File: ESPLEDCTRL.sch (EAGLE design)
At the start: 6 parts, among them J1 22-27-2031-03, X3 ZX62D-B-5PA8

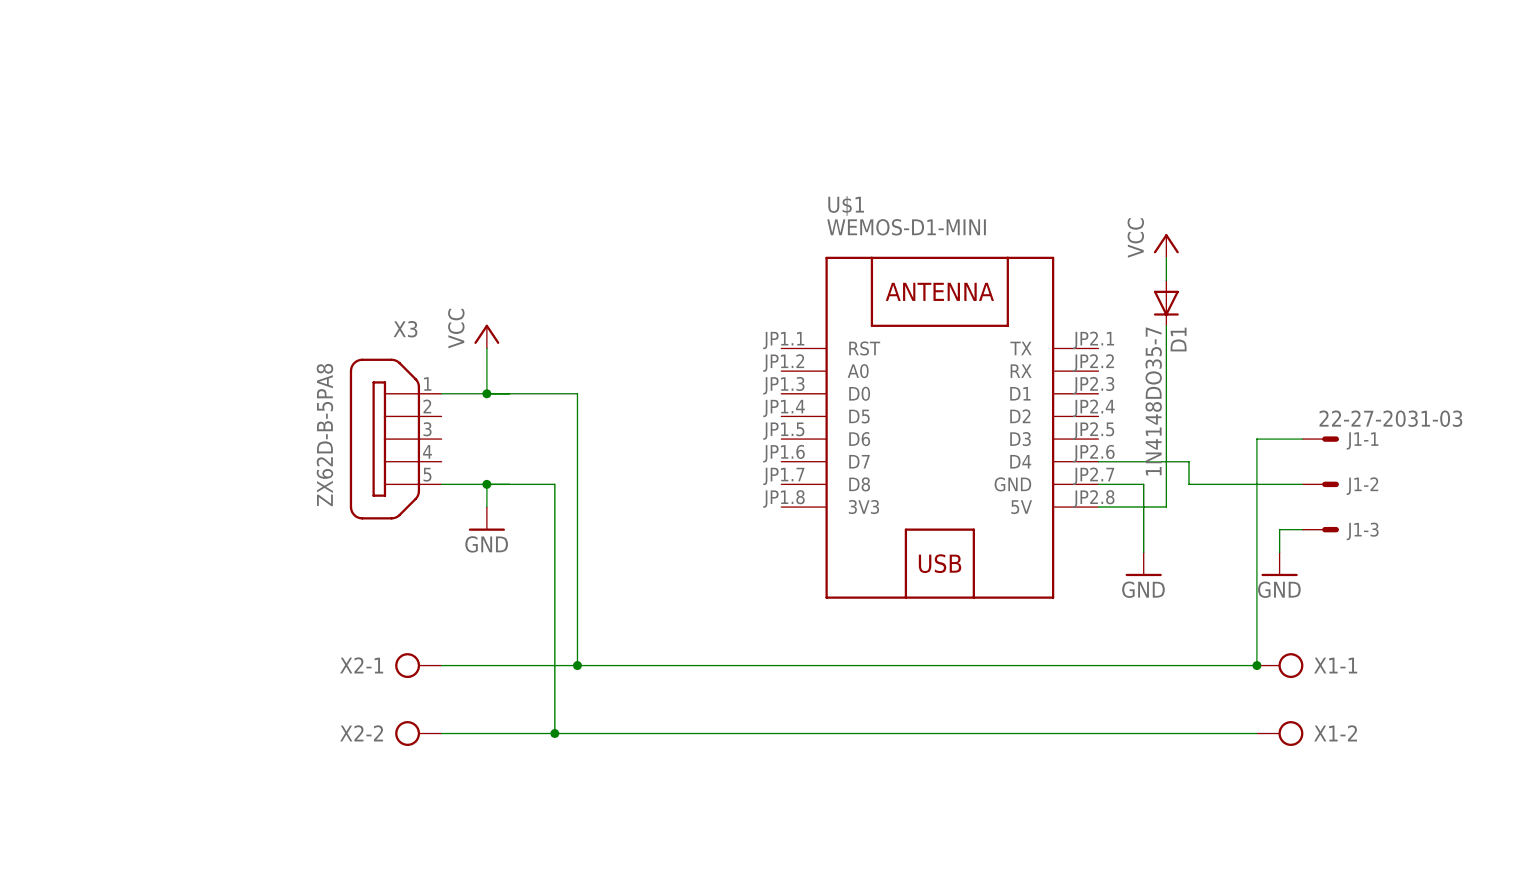
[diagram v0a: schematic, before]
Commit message: some changes
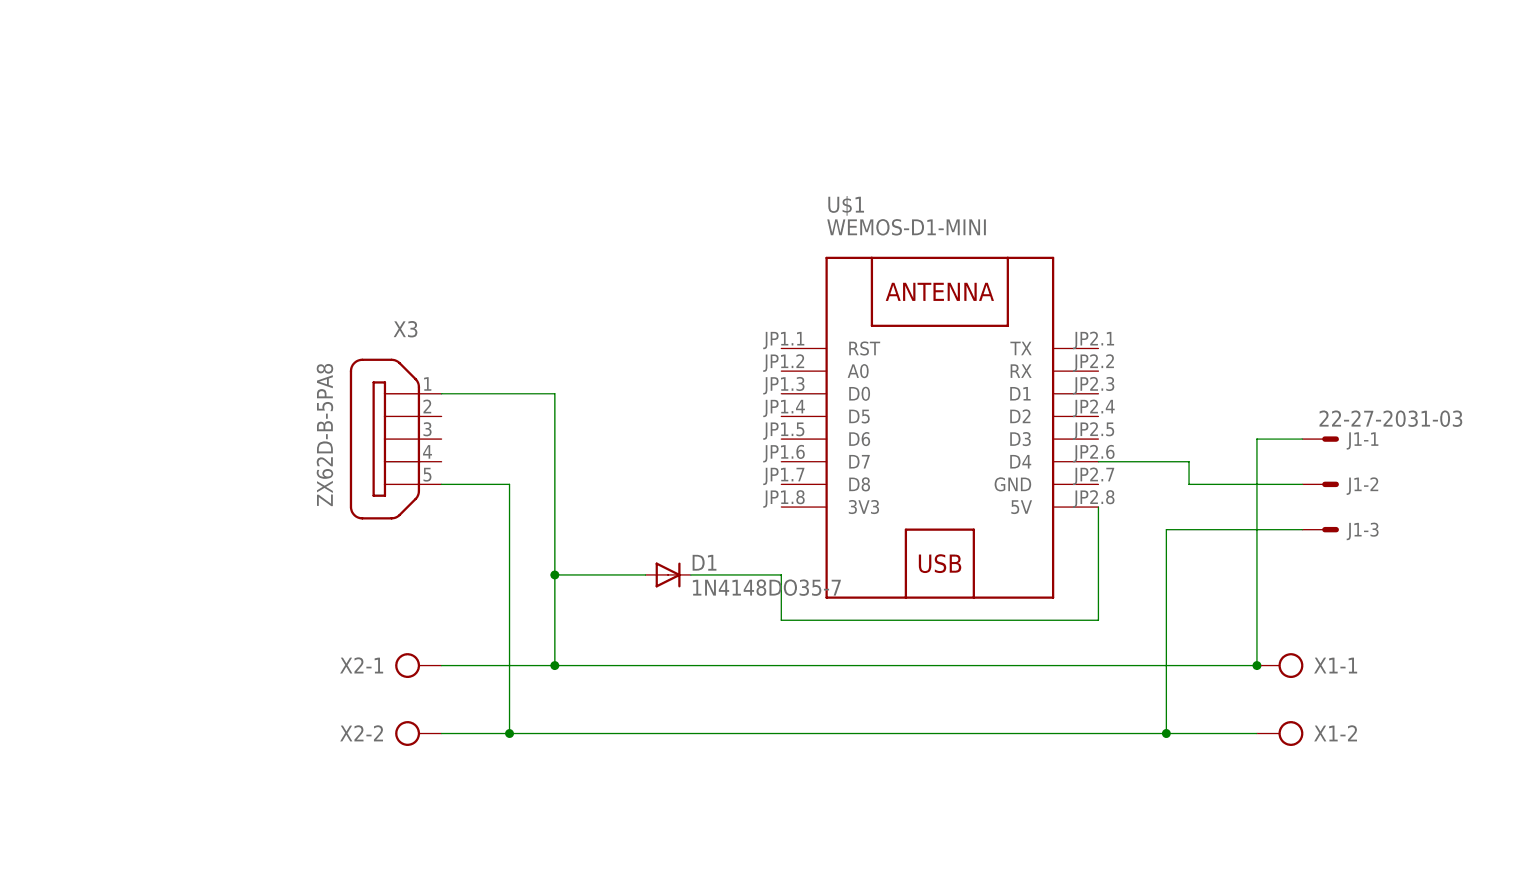
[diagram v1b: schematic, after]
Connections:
- net VCC renamed N$3
- removed net GND: J1-3.S, U$1.GND, X1-2.KL, X2-2.KL, X3G$1.5
- new net N$6: J1-3.S, X1-2.KL, X2-2.KL, X3G$1.5
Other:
- moved on the sheet: D1
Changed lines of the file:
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@@
 <?xml version="1.0" encoding="utf-8"?>
 <!DOCTYPE eagle SYSTEM "eagle.dtd">
-<eagle version="8.7.1">
+<eagle version="9.5.1">
 <drawing>
 <settings>
@@
 <parts>
 <part name="X3" library="zx62d-b-5pa8-oshpark_10" deviceset="ZX62D-B-5PA8" device=""/>
-<part name="P+1" library="supply1" library_urn="urn:adsk.eagle:library:371" deviceset="VCC" device=""/>
-<part name="GND1" library="supply1" library_urn="urn:adsk.eagle:library:371" deviceset="GND" device=""/>
 <part name="U$1" library="diy-modules" deviceset="WEMOS-D1-MINI" device=""/>
 <part name="X1" library="con-ptr500" library_urn="urn:adsk.eagle:library:181" deviceset="AK300/2" device="" package3d_urn="urn:adsk.eagle:package:9881/1"/>
 <part name="X2" library="con-ptr500" library_urn="urn:adsk.eagle:library:181" deviceset="AK300/2" device="" package3d_urn="urn:adsk.eagle:package:9881/1"/>
 <part name="J1" library="con-molex" library_urn="urn:adsk.eagle:library:165" deviceset="22-?-03" device="27-2031"/>
-<part name="GND2" library="supply1" library_urn="urn:adsk.eagle:library:371" deviceset="GND" device=""/>
-<part name="P+2" library="supply1" library_urn="urn:adsk.eagle:library:371" deviceset="VCC" device=""/>
-<part name="GND3" library="supply1" library_urn="urn:adsk.eagle:library:371" deviceset="GND" device=""/>
 <part name="D1" library="diode" library_urn="urn:adsk.eagle:library:210" deviceset="1N4148" device="DO35-7" package3d_urn="urn:adsk.eagle:package:43339/1"/>
 </parts>
@@
 <attribute name="VALUE" x="19.05" y="50.8" size="1.778" layer="96" font="vector" rot="MR90"/>
 </instance>
-<instance part="P+1" gate="VCC" x="38.1" y="71.12" smashed="yes">
-<attribute name="VALUE" x="35.56" y="68.58" size="1.778" layer="96" rot="R90"/>
-</instance>
-<instance part="GND1" gate="1" x="38.1" y="48.26" smashed="yes">
-<attribute name="VALUE" x="35.56" y="45.72" size="1.778" layer="96"/>
-</instance>
 <instance part="U$1" gate="G$1" x="88.9" y="58.42" smashed="yes">
 <attribute name="NAME" x="76.2" y="83.82" size="1.778" layer="95"/>
@@
 <attribute name="NAME" x="134.62" y="47.498" size="1.524" layer="95"/>
 </instance>
-<instance part="GND2" gate="1" x="127" y="43.18" smashed="yes">
-<attribute name="VALUE" x="124.46" y="40.64" size="1.778" layer="96"/>
-</instance>
-<instance part="P+2" gate="VCC" x="114.3" y="81.28" smashed="yes">
-<attribute name="VALUE" x="111.76" y="78.74" size="1.778" layer="96" rot="R90"/>
-</instance>
-<instance part="GND3" gate="1" x="111.76" y="43.18" smashed="yes">
-<attribute name="VALUE" x="109.22" y="40.64" size="1.778" layer="96"/>
-</instance>
-<instance part="D1" gate="G$1" x="114.3" y="73.66" rot="R270"/>
+<instance part="D1" gate="G$1" x="58.42" y="43.18" smashed="yes">
+<attribute name="NAME" x="60.96" y="43.6626" size="1.778" layer="95"/>
+<attribute name="VALUE" x="60.96" y="40.8686" size="1.778" layer="96"/>
+</instance>
 </instances>
 <busses>
 </busses>
 <nets>
-<net name="GND" class="0">
-<segment>
-<pinref part="GND1" gate="1" pin="GND"/>
-<wire x1="40.64" y1="53.34" x2="38.1" y2="53.34" width="0.1524" layer="91"/>
-<wire x1="38.1" y1="53.34" x2="38.1" y2="50.8" width="0.1524" layer="91"/>
-<junction x="38.1" y="53.34"/>
-<wire x1="38.1" y1="53.34" x2="33.02" y2="53.34" width="0.1524" layer="91"/>
-<pinref part="X3" gate="G$1" pin="5"/>
-<pinref part="X1" gate="-2" pin="KL"/>
-<wire x1="33.02" y1="25.4" x2="45.72" y2="25.4" width="0.1524" layer="91"/>
-<pinref part="X2" gate="-2" pin="KL"/>
-<wire x1="45.72" y1="25.4" x2="124.46" y2="25.4" width="0.1524" layer="91"/>
-<wire x1="45.72" y1="25.4" x2="45.72" y2="53.34" width="0.1524" layer="91"/>
-<wire x1="45.72" y1="53.34" x2="38.1" y2="53.34" width="0.1524" layer="91"/>
-<junction x="45.72" y="25.4"/>
-</segment>
-<segment>
-<pinref part="U$1" gate="G$1" pin="GND"/>
-<wire x1="106.68" y1="53.34" x2="111.76" y2="53.34" width="0.1524" layer="91"/>
-<wire x1="111.76" y1="53.34" x2="111.76" y2="45.72" width="0.1524" layer="91"/>
-<pinref part="GND3" gate="1" pin="GND"/>
-</segment>
-<segment>
-<pinref part="J1" gate="-3" pin="S"/>
-<pinref part="GND2" gate="1" pin="GND"/>
-<wire x1="129.54" y1="48.26" x2="127" y2="48.26" width="0.1524" layer="91"/>
-<wire x1="127" y1="48.26" x2="127" y2="45.72" width="0.1524" layer="91"/>
-</segment>
-</net>
-<net name="VCC" class="0">
-<segment>
-<pinref part="P+1" gate="VCC" pin="VCC"/>
-<wire x1="40.64" y1="63.5" x2="38.1" y2="63.5" width="0.1524" layer="91"/>
-<wire x1="38.1" y1="63.5" x2="38.1" y2="68.58" width="0.1524" layer="91"/>
-<junction x="38.1" y="63.5"/>
-<wire x1="38.1" y1="63.5" x2="33.02" y2="63.5" width="0.1524" layer="91"/>
-<pinref part="X3" gate="G$1" pin="1"/>
-<pinref part="X1" gate="-1" pin="KL"/>
-<pinref part="J1" gate="-1" pin="S"/>
-<wire x1="48.26" y1="33.02" x2="124.46" y2="33.02" width="0.1524" layer="91"/>
-<wire x1="129.54" y1="58.42" x2="124.46" y2="58.42" width="0.1524" layer="91"/>
-<wire x1="124.46" y1="58.42" x2="124.46" y2="33.02" width="0.1524" layer="91"/>
-<junction x="124.46" y="33.02"/>
-<wire x1="48.26" y1="33.02" x2="48.26" y2="63.5" width="0.1524" layer="91"/>
-<wire x1="48.26" y1="63.5" x2="38.1" y2="63.5" width="0.1524" layer="91"/>
-<pinref part="X2" gate="-1" pin="KL"/>
-<wire x1="48.26" y1="33.02" x2="33.02" y2="33.02" width="0.1524" layer="91"/>
-<junction x="48.26" y="33.02"/>
-</segment>
-<segment>
-<pinref part="P+2" gate="VCC" pin="VCC"/>
-<pinref part="D1" gate="G$1" pin="A"/>
-<wire x1="114.3" y1="76.2" x2="114.3" y2="78.74" width="0.1524" layer="91"/>
-</segment>
-</net>
 <net name="N$1" class="0">
 <segment>
@@
 </segment>
 </net>
+<net name="N$3" class="0">
+<segment>
+<pinref part="X1" gate="-1" pin="KL"/>
+<wire x1="33.02" y1="33.02" x2="45.72" y2="33.02" width="0.1524" layer="91"/>
+<pinref part="X2" gate="-1" pin="KL"/>
+<pinref part="X3" gate="G$1" pin="1"/>
+<wire x1="45.72" y1="33.02" x2="124.46" y2="33.02" width="0.1524" layer="91"/>
+<wire x1="33.02" y1="63.5" x2="45.72" y2="63.5" width="0.1524" layer="91"/>
+<wire x1="45.72" y1="63.5" x2="45.72" y2="43.18" width="0.1524" layer="91"/>
+<junction x="45.72" y="33.02"/>
+<pinref part="D1" gate="G$1" pin="A"/>
+<wire x1="45.72" y1="43.18" x2="45.72" y2="33.02" width="0.1524" layer="91"/>
+<wire x1="55.88" y1="43.18" x2="45.72" y2="43.18" width="0.1524" layer="91"/>
+<junction x="45.72" y="43.18"/>
+<pinref part="J1" gate="-1" pin="S"/>
+<wire x1="124.46" y1="33.02" x2="124.46" y2="58.42" width="0.1524" layer="91"/>
+<wire x1="124.46" y1="58.42" x2="129.54" y2="58.42" width="0.1524" layer="91"/>
+<junction x="124.46" y="33.02"/>
+</segment>
+</net>
 <net name="N$2" class="0">
 <segment>
+<pinref part="D1" gate="G$1" pin="C"/>
+<wire x1="60.96" y1="43.18" x2="71.12" y2="43.18" width="0.1524" layer="91"/>
+<wire x1="71.12" y1="43.18" x2="71.12" y2="38.1" width="0.1524" layer="91"/>
 <pinref part="U$1" gate="G$1" pin="5V"/>
-<wire x1="106.68" y1="50.8" x2="114.3" y2="50.8" width="0.1524" layer="91"/>
-<wire x1="114.3" y1="50.8" x2="114.3" y2="71.12" width="0.1524" layer="91"/>
-<pinref part="D1" gate="G$1" pin="C"/>
-</segment>
-</net>
+<wire x1="71.12" y1="38.1" x2="106.68" y2="38.1" width="0.1524" layer="91"/>
+<wire x1="106.68" y1="38.1" x2="106.68" y2="50.8" width="0.1524" layer="91"/>
+</segment>
+</net>
+<net name="N$6" class="0">
+<segment>
+<pinref part="X3" gate="G$1" pin="5"/>
+<wire x1="33.02" y1="53.34" x2="40.64" y2="53.34" width="0.1524" layer="91"/>
+<pinref part="X1" gate="-2" pin="KL"/>
+<pinref part="X2" gate="-2" pin="KL"/>
+<wire x1="33.02" y1="25.4" x2="40.64" y2="25.4" width="0.1524" layer="91"/>
+<pinref part="J1" gate="-3" pin="S"/>
+<wire x1="40.64" y1="25.4" x2="114.3" y2="25.4" width="0.1524" layer="91"/>
+<wire x1="114.3" y1="25.4" x2="124.46" y2="25.4" width="0.1524" layer="91"/>
+<wire x1="129.54" y1="48.26" x2="114.3" y2="48.26" width="0.1524" layer="91"/>
+<wire x1="114.3" y1="48.26" x2="114.3" y2="25.4" width="0.1524" layer="91"/>
+<junction x="114.3" y="25.4"/>
+<wire x1="40.64" y1="53.34" x2="40.64" y2="25.4" width="0.1524" layer="91"/>
+<junction x="40.64" y="25.4"/>
+</segment>
+</net>

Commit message: Alte Version
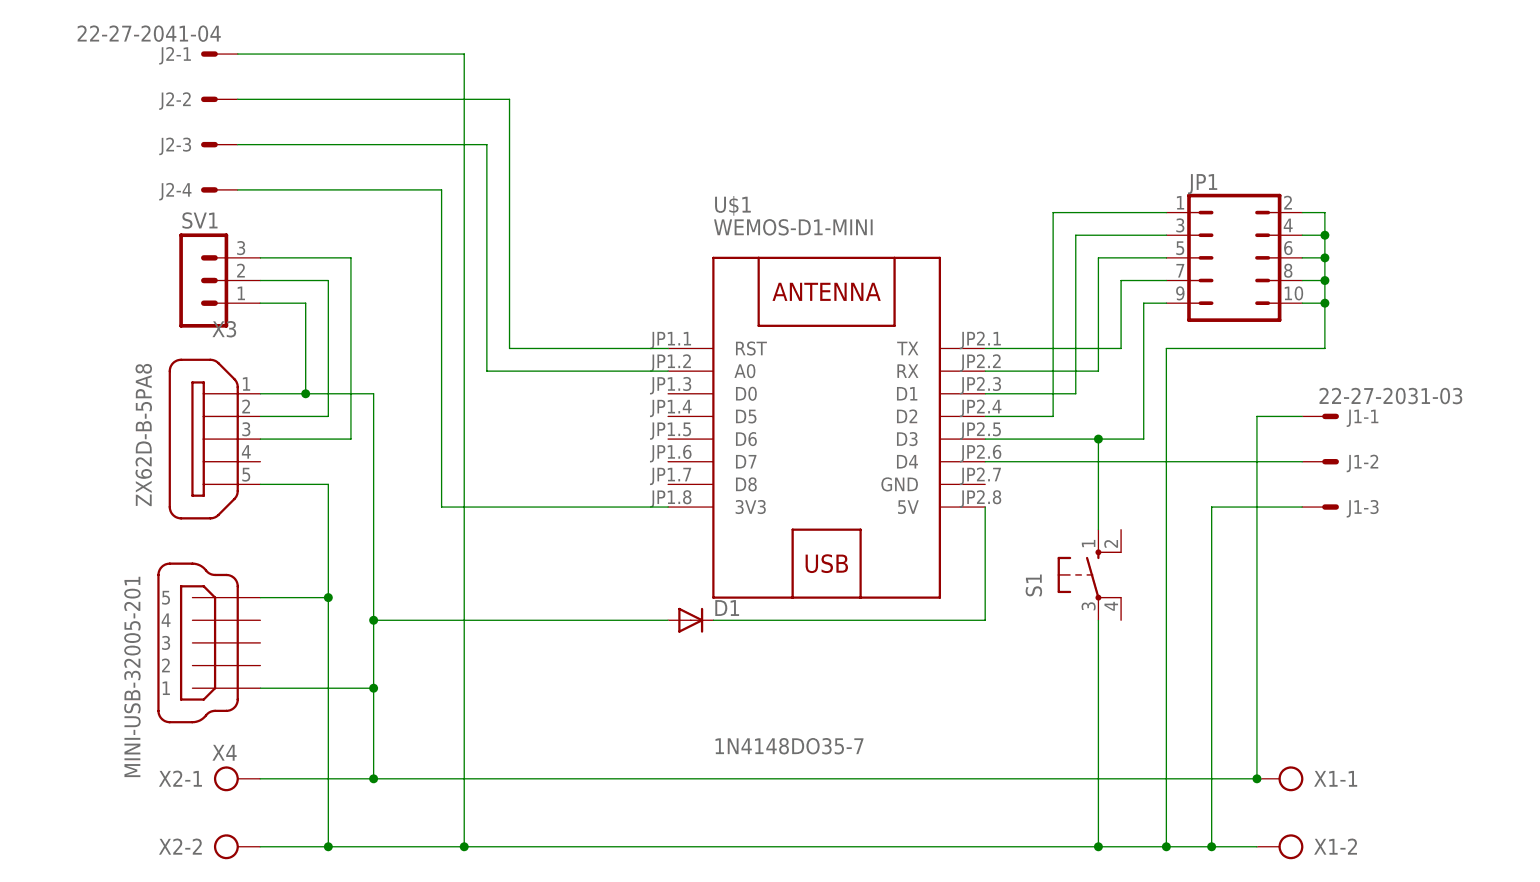
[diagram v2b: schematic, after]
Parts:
- added J2: 22-27-2041-04, con-molex:22-27-2041-04
- added JP1: (no value), jumper:JP5Q
- added S1: (no value), switch-omron:10-XX
- added SV1: (no value), con-lstb:MA03-1
- added X4: MINI-USB-32005-201, con-cypressindustries:MINI-USB-32005-201
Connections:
- new net N$10: J2-3.S, U$1.A0
- new net N$11: J1-3.S, J2-1.S, JP1.10, JP1.2, JP1.4, JP1.6, JP1.8, S1.P, X1-2.KL, X2-2.KL, X3G$1.5, X4.5
- new net N$12: J2-4.S, U$1.3V3
- new net N$13: D1.A, J1-1.S, SV1.1, X1-1.KL, X2-1.KL, X3G$1.1, X4.1
- new net N$14: SV1.3, X3G$1.3
- new net N$4: JP1.9, S1.S, U$1.D3
- new net N$5: JP1.1, U$1.D2
- new net N$7: JP1.3, U$1.D1
- new net N$8: JP1.5, U$1.RX
- new net N$9: JP1.7, U$1.TX
- net N$3: now also SV1.2, X3G$1.2; no longer D1.A, J1-1.S, X1-1.KL, X2-1.KL, X3G$1.1
- net N$6: now also J2-2.S, U$1.RST; no longer J1-3.S, X1-2.KL, X2-2.KL, X3G$1.5
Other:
- moved on the sheet: D1, J1-1, J1-2, J1-3, U$1, X1-1, X1-2, X2-1, X2-2, X3
